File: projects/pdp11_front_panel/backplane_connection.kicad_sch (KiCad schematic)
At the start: 1 part

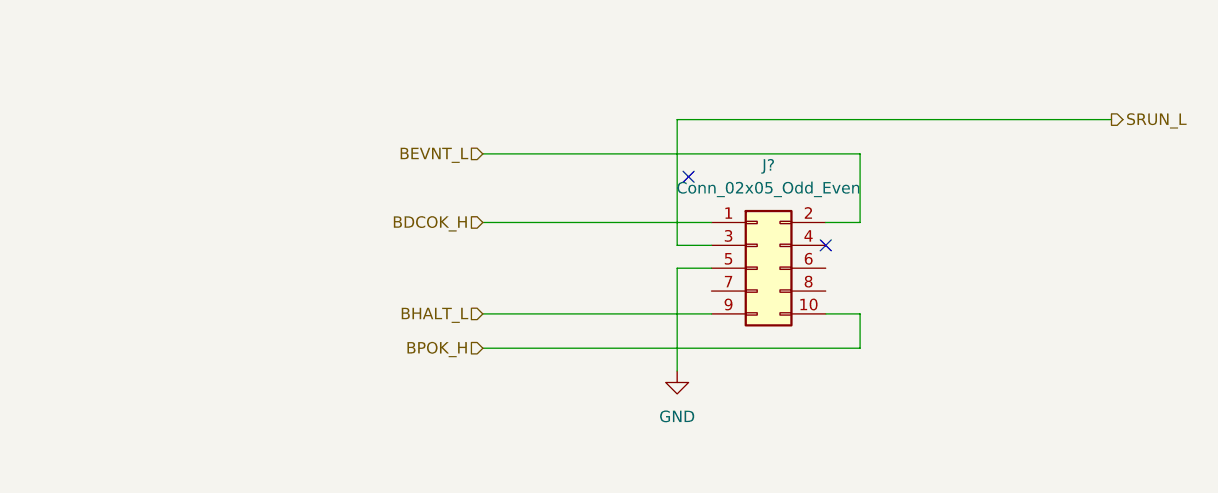
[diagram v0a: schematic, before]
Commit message: .
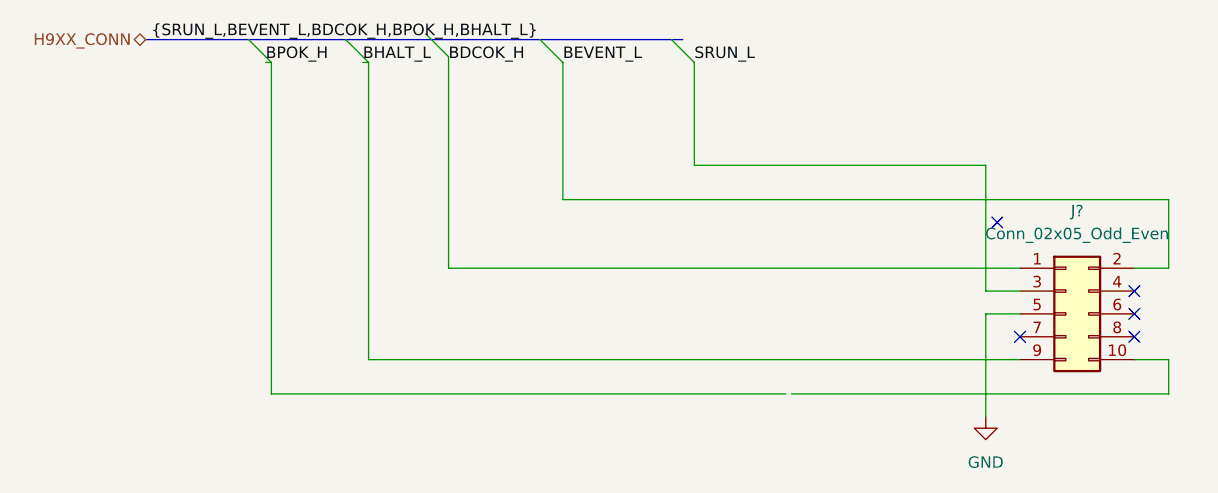
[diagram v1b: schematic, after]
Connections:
- net BPOK_H: no longer J?.10 (Pin_10)
- net BEVNT_L renamed BEVENT_L
- no-connect marks 2 -> 5
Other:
- moved on the sheet: J?
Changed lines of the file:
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@@
 (kicad_sch (version 20211123) (generator eeschema)
   (paper "A4")
-  (no_connect (at 88.9 101.6))
-  (no_connect (at 104.14 109.22))
-  (wire (pts (xy 87.63 111.76) (xy 91.44 111.76))
+  (no_connect (at 123.19 106.68))
+  (no_connect (at 138.43 114.3))
+  (no_connect (at 138.43 116.84))
+  (no_connect (at 138.43 119.38))
+  (no_connect (at 125.73 119.38))
+  (bus_entry (at 50.8 86.36) (size 2.54 2.54)
     (stroke (width 0) (type default) (color 0 0 0 0))
   )
-  (wire (pts (xy 66.04 116.84) (xy 91.44 116.84))
+  (bus_entry (at 86.995 86.36) (size 2.54 2.54)
     (stroke (width 0) (type default) (color 0 0 0 0))
   )
-  (wire (pts (xy 107.95 116.84) (xy 104.14 116.84))
+  (bus_entry (at 59.69 85.725) (size 2.54 2.54)
     (stroke (width 0) (type default) (color 0 0 0 0))
   )
-  (wire (pts (xy 104.14 106.68) (xy 107.95 106.68))
+  (bus_entry (at 40.005 86.36) (size 2.54 2.54)
     (stroke (width 0) (type default) (color 0 0 0 0))
   )
-  (wire (pts (xy 107.95 106.68) (xy 107.95 99.06))
+  (bus_entry (at 72.39 86.36) (size 2.54 2.54)
     (stroke (width 0) (type default) (color 0 0 0 0))
   )
-  (wire (pts (xy 87.63 109.22) (xy 91.44 109.22))
+  (wire (pts (xy 52.705 88.9) (xy 53.34 88.9))
     (stroke (width 0) (type default) (color 0 0 0 0))
   )
-  (wire (pts (xy 107.95 120.65) (xy 107.95 116.84))
+  (wire (pts (xy 121.92 116.84) (xy 125.73 116.84))
     (stroke (width 0) (type default) (color 0 0 0 0))
   )
-  (wire (pts (xy 107.95 99.06) (xy 66.04 99.06))
+  (wire (pts (xy 53.34 121.92) (xy 125.73 121.92))
     (stroke (width 0) (type default) (color 0 0 0 0))
   )
-  (wire (pts (xy 87.63 95.25) (xy 87.63 109.22))
+  (wire (pts (xy 142.24 121.92) (xy 138.43 121.92))
     (stroke (width 0) (type default) (color 0 0 0 0))
   )
-  (wire (pts (xy 87.63 111.76) (xy 87.63 123.19))
+  (wire (pts (xy 138.43 111.76) (xy 142.24 111.76))
     (stroke (width 0) (type default) (color 0 0 0 0))
   )
-  (wire (pts (xy 66.04 120.65) (xy 107.95 120.65))
+  (wire (pts (xy 142.24 111.76) (xy 142.24 104.14))
     (stroke (width 0) (type default) (color 0 0 0 0))
   )
-  (wire (pts (xy 135.89 95.25) (xy 87.63 95.25))
+  (wire (pts (xy 74.93 104.14) (xy 142.24 104.14))
     (stroke (width 0) (type default) (color 0 0 0 0))
   )
-  (wire (pts (xy 66.04 106.68) (xy 91.44 106.68))
+  (wire (pts (xy 53.34 121.92) (xy 53.34 88.9))
+    (stroke (width 0) (type default) (color 0 0 0 0))
+  )
+  (bus (pts (xy 28.575 86.36) (xy 40.005 86.36))
+    (stroke (width 0) (type default) (color 0 0 0 0))
+  )
+  (bus (pts (xy 40.005 86.36) (xy 50.8 86.36))
+    (stroke (width 0) (type default) (color 0 0 0 0))
+  )
+  (wire (pts (xy 121.92 114.3) (xy 125.73 114.3))
+    (stroke (width 0) (type default) (color 0 0 0 0))
+  )
+  (wire (pts (xy 89.535 88.9) (xy 89.535 100.33))
+    (stroke (width 0) (type default) (color 0 0 0 0))
+  )
+  (wire (pts (xy 142.24 125.73) (xy 142.24 121.92))
+    (stroke (width 0) (type default) (color 0 0 0 0))
+  )
+  (wire (pts (xy 42.545 125.73) (xy 42.545 88.9))
+    (stroke (width 0) (type default) (color 0 0 0 0))
+  )
+  (wire (pts (xy 62.23 88.265) (xy 62.23 111.76))
+    (stroke (width 0) (type default) (color 0 0 0 0))
+  )
+  (wire (pts (xy 42.545 125.73) (xy 99.695 125.73))
+    (stroke (width 0) (type default) (color 0 0 0 0))
+  )
+  (wire (pts (xy 121.92 100.33) (xy 121.92 114.3))
+    (stroke (width 0) (type default) (color 0 0 0 0))
+  )
+  (wire (pts (xy 89.535 100.33) (xy 121.92 100.33))
+    (stroke (width 0) (type default) (color 0 0 0 0))
+  )
+  (bus (pts (xy 72.39 86.36) (xy 86.995 86.36))
+    (stroke (width 0) (type default) (color 0 0 0 0))
+  )
+  (wire (pts (xy 121.92 116.84) (xy 121.92 128.27))
+    (stroke (width 0) (type default) (color 0 0 0 0))
+  )
+  (wire (pts (xy 41.91 88.9) (xy 42.545 88.9))
+    (stroke (width 0) (type default) (color 0 0 0 0))
+  )
+  (wire (pts (xy 100.33 125.73) (xy 142.24 125.73))
+    (stroke (width 0) (type default) (color 0 0 0 0))
+  )
+  (bus (pts (xy 86.995 86.36) (xy 88.265 86.36))
+    (stroke (width 0) (type default) (color 0 0 0 0))
+  )
+  (bus (pts (xy 50.8 86.36) (xy 72.39 86.36))
+    (stroke (width 0) (type default) (color 0 0 0 0))
+  )
+  (wire (pts (xy 74.93 88.9) (xy 74.93 104.14))
+    (stroke (width 0) (type default) (color 0 0 0 0))
+  )
+  (wire (pts (xy 62.23 111.76) (xy 125.73 111.76))
     (stroke (width 0) (type default) (color 0 0 0 0))
   )
@@
     )
   )
-  (hierarchical_label "BDCOK_H" (shape input) (at 66.04 106.68 180)
-    (effects (font (size 1.27 1.27)) (justify right))
+  (label "SRUN_L" (at 89.535 88.9 0)
+    (effects (font (size 1.27 1.27)) (justify left bottom))
   )
-  (hierarchical_label "SRUN_L" (shape output) (at 135.89 95.25 0)
-    (effects (font (size 1.27 1.27)) (justify left))
+  (label "{SRUN_L,BEVENT_L,BDCOK_H,BPOK_H,BHALT_L}" (at 29.21 86.36 0)
+    (effects (font (size 1.27 1.27)) (justify left bottom))
   )
-  (hierarchical_label "BHALT_L" (shape input) (at 66.04 116.84 180)
-    (effects (font (size 1.27 1.27)) (justify right))
+  (label "BDCOK_H" (at 62.23 88.9 0)
+    (effects (font (size 1.27 1.27)) (justify left bottom))
   )
-  (hierarchical_label "BPOK_H" (shape input) (at 66.04 120.65 180)
-    (effects (font (size 1.27 1.27)) (justify right))
+  (label "BHALT_L" (at 52.705 88.9 0)
+    (effects (font (size 1.27 1.27)) (justify left bottom))
+  )
+  (label "BEVENT_L" (at 74.93 88.9 0)
+    (effects (font (size 1.27 1.27)) (justify left bottom))
+  )
+  (label "BPOK_H" (at 41.91 88.9 0)
+    (effects (font (size 1.27 1.27)) (justify left bottom))
   )
-  (hierarchical_label "BEVNT_L" (shape input) (at 66.04 99.06 180)
+  (hierarchical_label "H9XX_CONN" (shape bidirectional) (at 28.575 86.36 180)
     (effects (font (size 1.27 1.27)) (justify right))
   )
-  (symbol (lib_id "power:GND") (at 87.63 123.19 0) (unit 1)
+  (symbol (lib_id "power:GND") (at 121.92 128.27 0) (unit 1)
     (in_bom yes) (on_board yes) (fields_autoplaced)
-    (property "Reference" "#PWR?" (id 0) (at 87.63 129.54 0)
+    (property "Reference" "#PWR?" (id 0) (at 121.92 134.62 0)
       (effects (font (size 1.27 1.27)) hide)
     )
-    (property "Value" "GND" (id 1) (at 87.63 128.27 0))
-    (property "Footprint" "" (id 2) (at 87.63 123.19 0)
+    (property "Value" "GND" (id 1) (at 121.92 133.35 0))
+    (property "Footprint" "" (id 2) (at 121.92 128.27 0)
       (effects (font (size 1.27 1.27)) hide)
     )
-    (property "Datasheet" "" (id 3) (at 87.63 123.19 0)
+    (property "Datasheet" "" (id 3) (at 121.92 128.27 0)
       (effects (font (size 1.27 1.27)) hide)
     )
     (pin "1")
   )
-  (symbol (lib_id "Connector_Generic:Conn_02x05_Odd_Even") (at 96.52 111.76 0) (unit 1)
+  (symbol (lib_id "Connector_Generic:Conn_02x05_Odd_Even") (at 130.81 116.84 0) (unit 1)
     (in_bom yes) (on_board yes) (fields_autoplaced)
-    (property "Reference" "J?" (id 0) (at 97.79 100.33 0))
-    (property "Value" "Conn_02x05_Odd_Even" (id 1) (at 97.79 102.87 0))
-    (property "Footprint" "" (id 2) (at 96.52 111.76 0)
+    (property "Reference" "J?" (id 0) (at 132.08 105.41 0))
+    (property "Value" "Conn_02x05_Odd_Even" (id 1) (at 132.08 107.95 0))
+    (property "Footprint" "" (id 2) (at 130.81 116.84 0)
       (effects (font (size 1.27 1.27)) hide)
     )
-    (property "Datasheet" "~" (id 3) (at 96.52 111.76 0)
+    (property "Datasheet" "~" (id 3) (at 130.81 116.84 0)
       (effects (font (size 1.27 1.27)) hide)
     )
